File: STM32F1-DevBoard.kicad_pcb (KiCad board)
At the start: 2 copper layers, 20.3 x 50.8 mm, 39 parts, among them J1 USB_C_Receptacle_USB2.0, SW1 SW_Push, SW2 SW_Push, U1 STM32F103C8T6, U2 AMS1117-3.3, U3 W25Q32JVSS

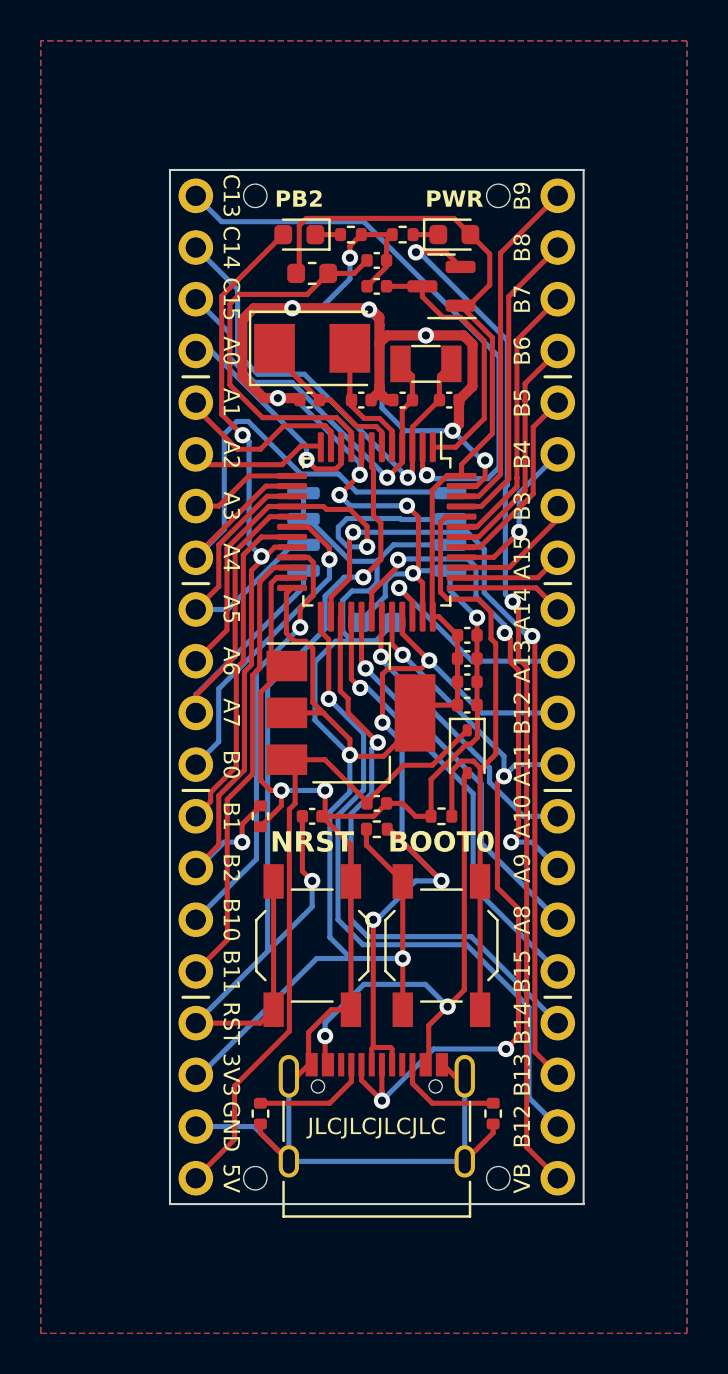
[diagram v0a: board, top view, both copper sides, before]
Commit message: Add files via upload
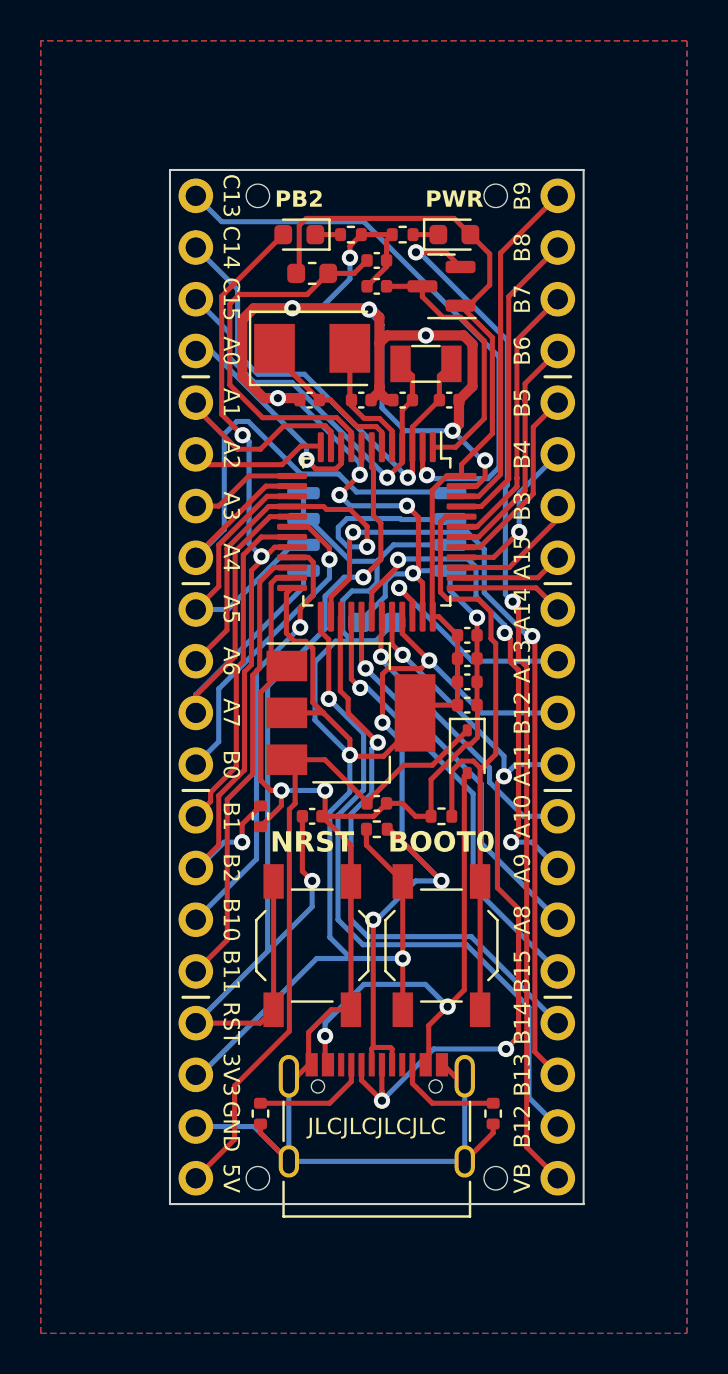
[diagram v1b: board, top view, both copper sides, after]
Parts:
- moved H1 0.13 mm to (131.3, 125.7)
- moved H2 0.13 mm to (131.3, 77.5)
- moved H3 0.13 mm to (143.0, 77.5)
- moved H4 0.13 mm to (143.0, 125.7)
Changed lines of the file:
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@@
   )
   (footprint "MountingHole:MountingHole_2.2mm_M2" (layer "F.Cu")
-    (at 131.191 77.47)
+    (at 131.318 77.47)
     (descr "Mounting Hole 2.2mm, no annular, M2")
     (tags "mounting hole 2.2mm no annular m2")
@@
   )
   (footprint "MountingHole:MountingHole_2.2mm_M2" (layer "F.Cu")
-    (at 143.129 77.47)
+    (at 143.002 77.47)
     (descr "Mounting Hole 2.2mm, no annular, M2")
     (tags "mounting hole 2.2mm no annular m2")
@@
   )
   (footprint "MountingHole:MountingHole_2.2mm_M2" (layer "F.Cu")
-    (at 143.129 125.73)
+    (at 143.002 125.73)
     (descr "Mounting Hole 2.2mm, no annular, M2")
     (tags "mounting hole 2.2mm no annular m2")
@@
   )
   (footprint "MountingHole:MountingHole_2.2mm_M2" (layer "F.Cu")
-    (at 131.191 125.73)
+    (at 131.318 125.73)
     (descr "Mounting Hole 2.2mm, no annular, M2")
     (tags "mounting hole 2.2mm no annular m2")
